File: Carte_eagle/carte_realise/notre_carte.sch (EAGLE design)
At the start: 14 parts, among them CON1 CON-1X2-SPOX-M-2.50, CON2 CON-1X2-SPOX-M-2.50, U1 DOGM163

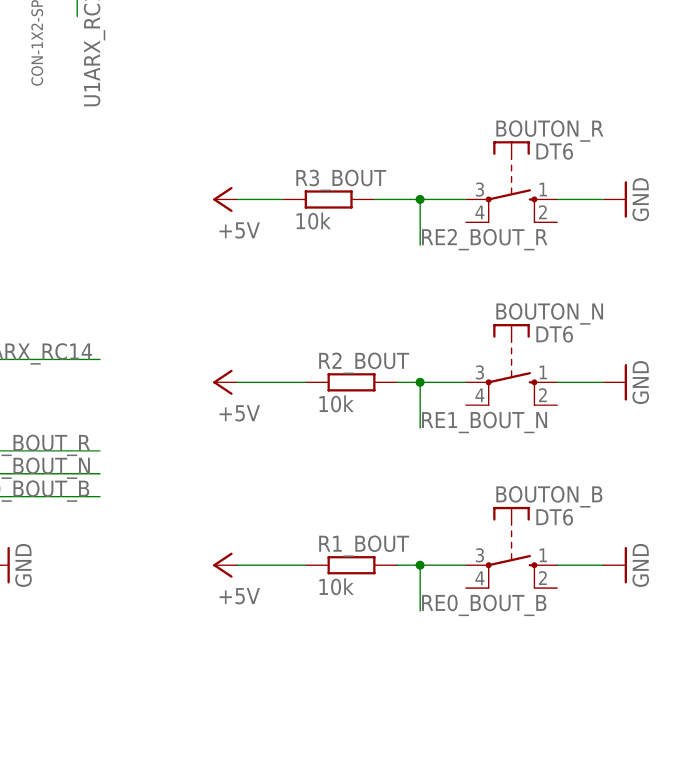
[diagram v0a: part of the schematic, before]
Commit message: mise a jour de la carte et board
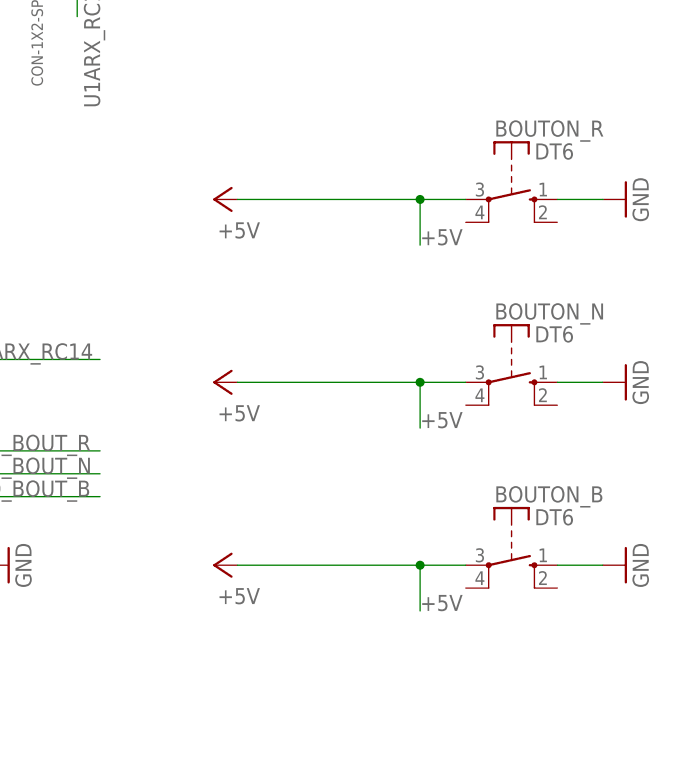
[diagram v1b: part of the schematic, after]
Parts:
- removed R1_BOUT, R2_BOUT, R3_BOUT: 10k, rcl:R-EU_0207/10
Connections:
- net +5V: now also BOUTON_B.P, BOUTON_N.P, BOUTON_R.P; no longer R1_BOUT.1, R2_BOUT.1, R3_BOUT.1
- net RE0_BOUT_B: no longer BOUTON_B.P, R1_BOUT.2
- net RE1_BOUT_N: no longer BOUTON_N.P, R2_BOUT.2
- net RE2_BOUT_R: no longer BOUTON_R.P, R3_BOUT.2
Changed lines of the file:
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@@
 <part name="BOUTON_N" library="switch-misc" deviceset="DT" device="6"/>
 <part name="BOUTON_R" library="switch-misc" deviceset="DT" device="6"/>
-<part name="R1_BOUT" library="rcl" deviceset="R-EU_" device="0207/10" value="10k"/>
-<part name="R2_BOUT" library="rcl" deviceset="R-EU_" device="0207/10" value="10k"/>
-<part name="R3_BOUT" library="rcl" deviceset="R-EU_" device="0207/10" value="10k"/>
 <part name="R_RETRO" library="rcl" deviceset="R-EU_" device="0207/15" value="33"/>
 <part name="GND5" library="supply1" deviceset="GND" device=""/>
@@
 <instance part="BOUTON_N" gate="1" x="182.88" y="63.5" rot="R270"/>
 <instance part="BOUTON_R" gate="1" x="182.88" y="83.82" rot="R270"/>
-<instance part="R1_BOUT" gate="G$1" x="165.1" y="43.18"/>
-<instance part="R2_BOUT" gate="G$1" x="165.1" y="63.5"/>
-<instance part="R3_BOUT" gate="G$1" x="162.56" y="83.82"/>
 <instance part="R_RETRO" gate="G$1" x="12.7" y="40.64" rot="R90"/>
 <instance part="GND5" gate="1" x="12.7" y="25.4"/>
@@
 <segment>
 <pinref part="P+6" gate="1" pin="+5V"/>
-<pinref part="R3_BOUT" gate="G$1" pin="1"/>
-<wire x1="152.4" y1="83.82" x2="157.48" y2="83.82" width="0.1524" layer="91"/>
+<pinref part="BOUTON_R" gate="1" pin="P"/>
+<wire x1="172.72" y1="83.82" x2="177.8" y2="83.82" width="0.1524" layer="91"/>
+<junction x="172.72" y="83.82"/>
+<wire x1="172.72" y1="78.74" x2="172.72" y2="83.82" width="0.1524" layer="91"/>
+<label x="172.72" y="78.74" size="1.778" layer="95"/>
+<wire x1="172.72" y1="83.82" x2="152.4" y2="83.82" width="0.1524" layer="91"/>
 </segment>
 <segment>
 <pinref part="P+7" gate="1" pin="+5V"/>
-<pinref part="R2_BOUT" gate="G$1" pin="1"/>
-<wire x1="152.4" y1="63.5" x2="160.02" y2="63.5" width="0.1524" layer="91"/>
+<pinref part="BOUTON_N" gate="1" pin="P"/>
+<wire x1="172.72" y1="63.5" x2="177.8" y2="63.5" width="0.1524" layer="91"/>
+<wire x1="172.72" y1="58.42" x2="172.72" y2="63.5" width="0.1524" layer="91"/>
+<junction x="172.72" y="63.5"/>
+<label x="172.72" y="58.42" size="1.778" layer="95"/>
+<wire x1="172.72" y1="63.5" x2="152.4" y2="63.5" width="0.1524" layer="91"/>
 </segment>
 <segment>
 <pinref part="P+8" gate="1" pin="+5V"/>
-<pinref part="R1_BOUT" gate="G$1" pin="1"/>
-<wire x1="152.4" y1="43.18" x2="160.02" y2="43.18" width="0.1524" layer="91"/>
+<pinref part="BOUTON_B" gate="1" pin="P"/>
+<wire x1="172.72" y1="43.18" x2="177.8" y2="43.18" width="0.1524" layer="91"/>
+<wire x1="172.72" y1="38.1" x2="172.72" y2="43.18" width="0.1524" layer="91"/>
+<junction x="172.72" y="43.18"/>
+<label x="172.72" y="38.1" size="1.778" layer="95"/>
+<wire x1="172.72" y1="43.18" x2="152.4" y2="43.18" width="0.1524" layer="91"/>
 </segment>
 <segment>
@@
 <label x="121.92" y="55.88" size="1.778" layer="95"/>
 </segment>
-<segment>
-<pinref part="BOUTON_R" gate="1" pin="P"/>
-<pinref part="R3_BOUT" gate="G$1" pin="2"/>
-<wire x1="167.64" y1="83.82" x2="172.72" y2="83.82" width="0.1524" layer="91"/>
-<wire x1="172.72" y1="83.82" x2="177.8" y2="83.82" width="0.1524" layer="91"/>
-<junction x="172.72" y="83.82"/>
-<wire x1="172.72" y1="78.74" x2="172.72" y2="83.82" width="0.1524" layer="91"/>
-<label x="172.72" y="78.74" size="1.778" layer="95"/>
-</segment>
 </net>
 <net name="U1ATX_RC13" class="0">
@@
 <label x="121.92" y="53.34" size="1.778" layer="95"/>
 </segment>
-<segment>
-<pinref part="R2_BOUT" gate="G$1" pin="2"/>
-<pinref part="BOUTON_N" gate="1" pin="P"/>
-<wire x1="170.18" y1="63.5" x2="172.72" y2="63.5" width="0.1524" layer="91"/>
-<wire x1="172.72" y1="63.5" x2="177.8" y2="63.5" width="0.1524" layer="91"/>
-<wire x1="172.72" y1="58.42" x2="172.72" y2="63.5" width="0.1524" layer="91"/>
-<junction x="172.72" y="63.5"/>
-<label x="172.72" y="58.42" size="1.778" layer="95"/>
-</segment>
 </net>
 <net name="RE0_BOUT_B" class="0">
@@
 <label x="121.92" y="50.8" size="1.778" layer="95"/>
 </segment>
-<segment>
-<pinref part="R1_BOUT" gate="G$1" pin="2"/>
-<pinref part="BOUTON_B" gate="1" pin="P"/>
-<wire x1="170.18" y1="43.18" x2="172.72" y2="43.18" width="0.1524" layer="91"/>
-<wire x1="172.72" y1="43.18" x2="177.8" y2="43.18" width="0.1524" layer="91"/>
-<wire x1="172.72" y1="38.1" x2="172.72" y2="43.18" width="0.1524" layer="91"/>
-<junction x="172.72" y="43.18"/>
-<label x="172.72" y="38.1" size="1.778" layer="95"/>
-</segment>
-</net>
+</net>
